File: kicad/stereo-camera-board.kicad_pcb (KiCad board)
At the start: 4 copper layers, 57 x 70 mm, 86 parts, among them IC1 ZLDO1117G33TA, IC2 MCP1700T-2502E/TT, IC3 SN74LVC1T45DCKR, IC4 SN74LVC1T45DCKR, IC5 SN74LVC1T45DCKR, T1 2n2222a, T2 2N2907A, U1 GSB311231HR, U2 ATXMEGA256A3-AU, U3 MAX3207E, U4 MPU-9250

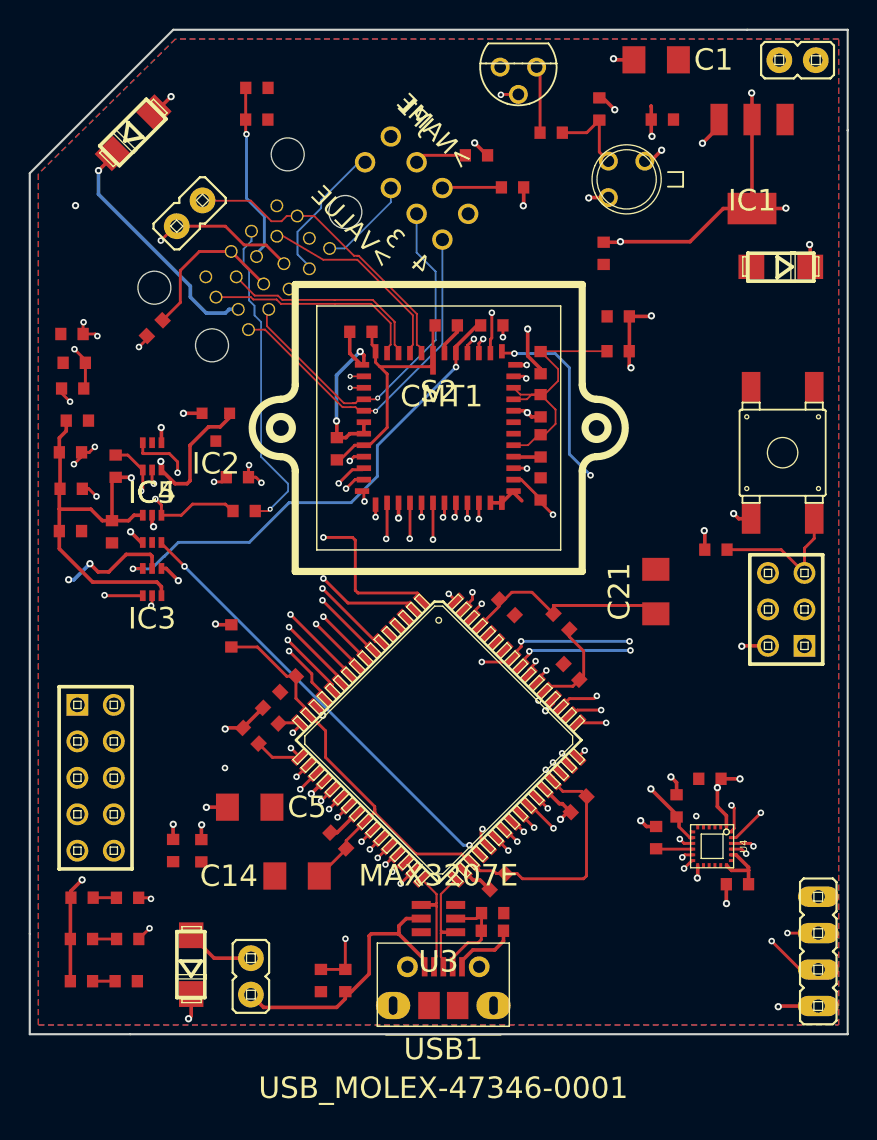
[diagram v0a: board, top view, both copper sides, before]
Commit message: Cleaned up module references for silk screen.
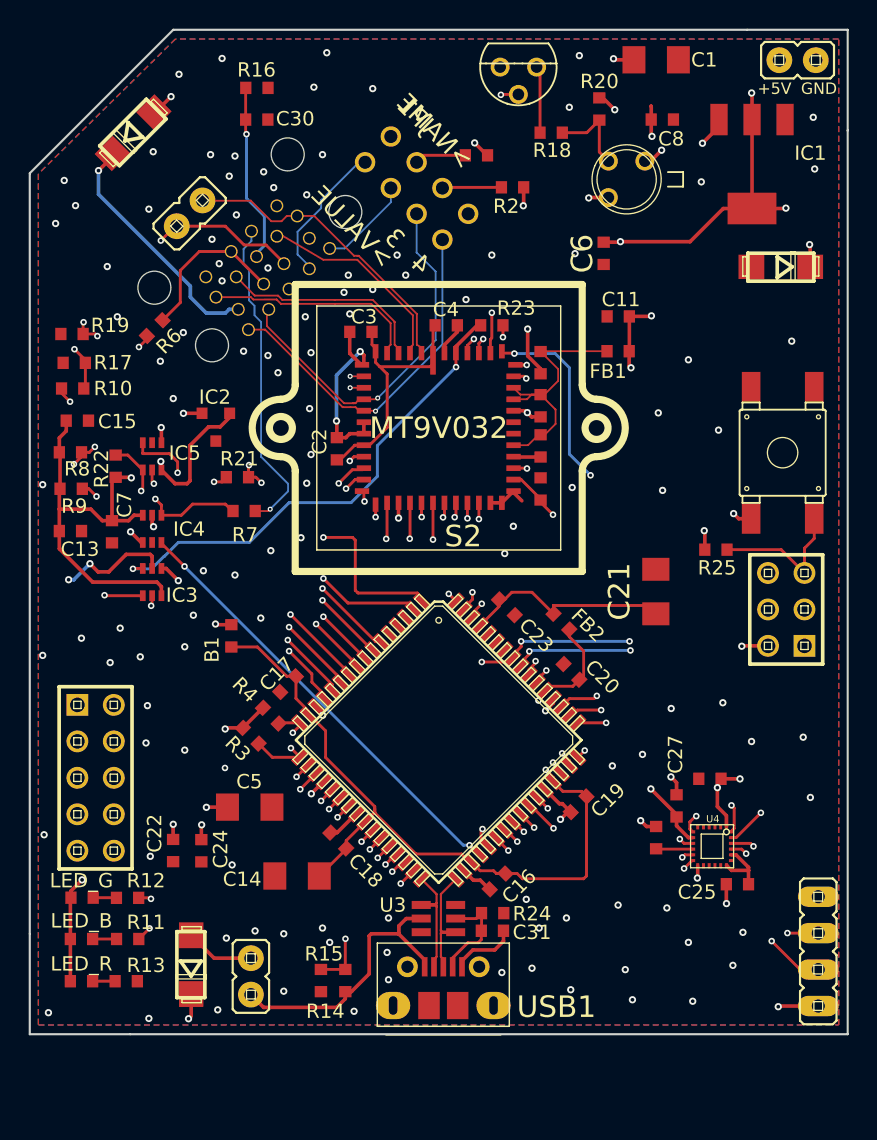
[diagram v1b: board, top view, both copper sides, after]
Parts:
- FSM4JSMA-SMD: renamed from Reset; value FSM4JSMA-SMD -> RESET
- JP3: value AVR-JTAG-10 -> JTAG
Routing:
- net N-0000067: track 14.9 -> 16.2 mm
- net (no net): track 1.19 -> 1.29 mm, vias 0 -> 109
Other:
- board text added: "+5V"
- board text added: "GND"
